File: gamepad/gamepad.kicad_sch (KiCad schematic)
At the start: 33 parts, among them J1 Conn_01x02_Socket, SW1 SW_SPDT, SW2 SW_Push, SW3 SW_Push, SW4 SW_Push, SW5 SW_Push, SW6 SW_Push, SW7 SW_Push, U1 NE555P

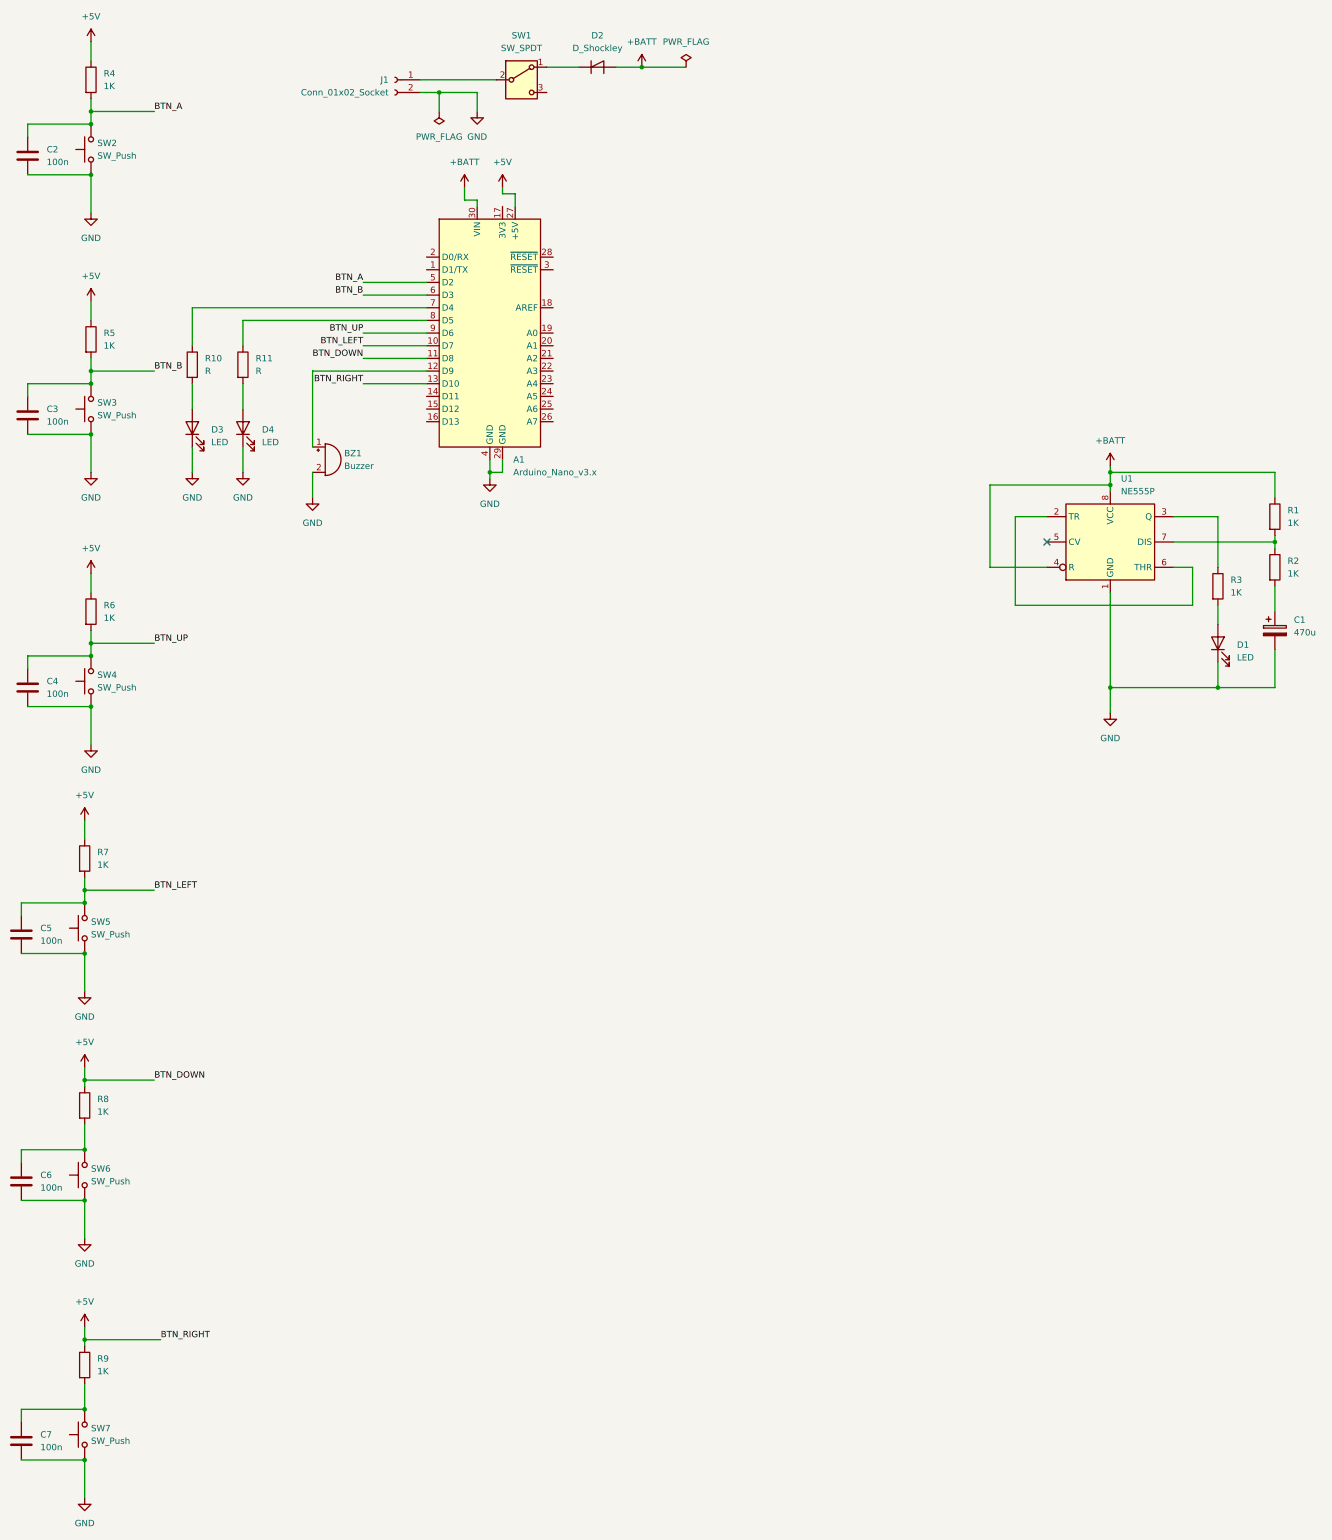
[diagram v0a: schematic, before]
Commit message: schematic is done
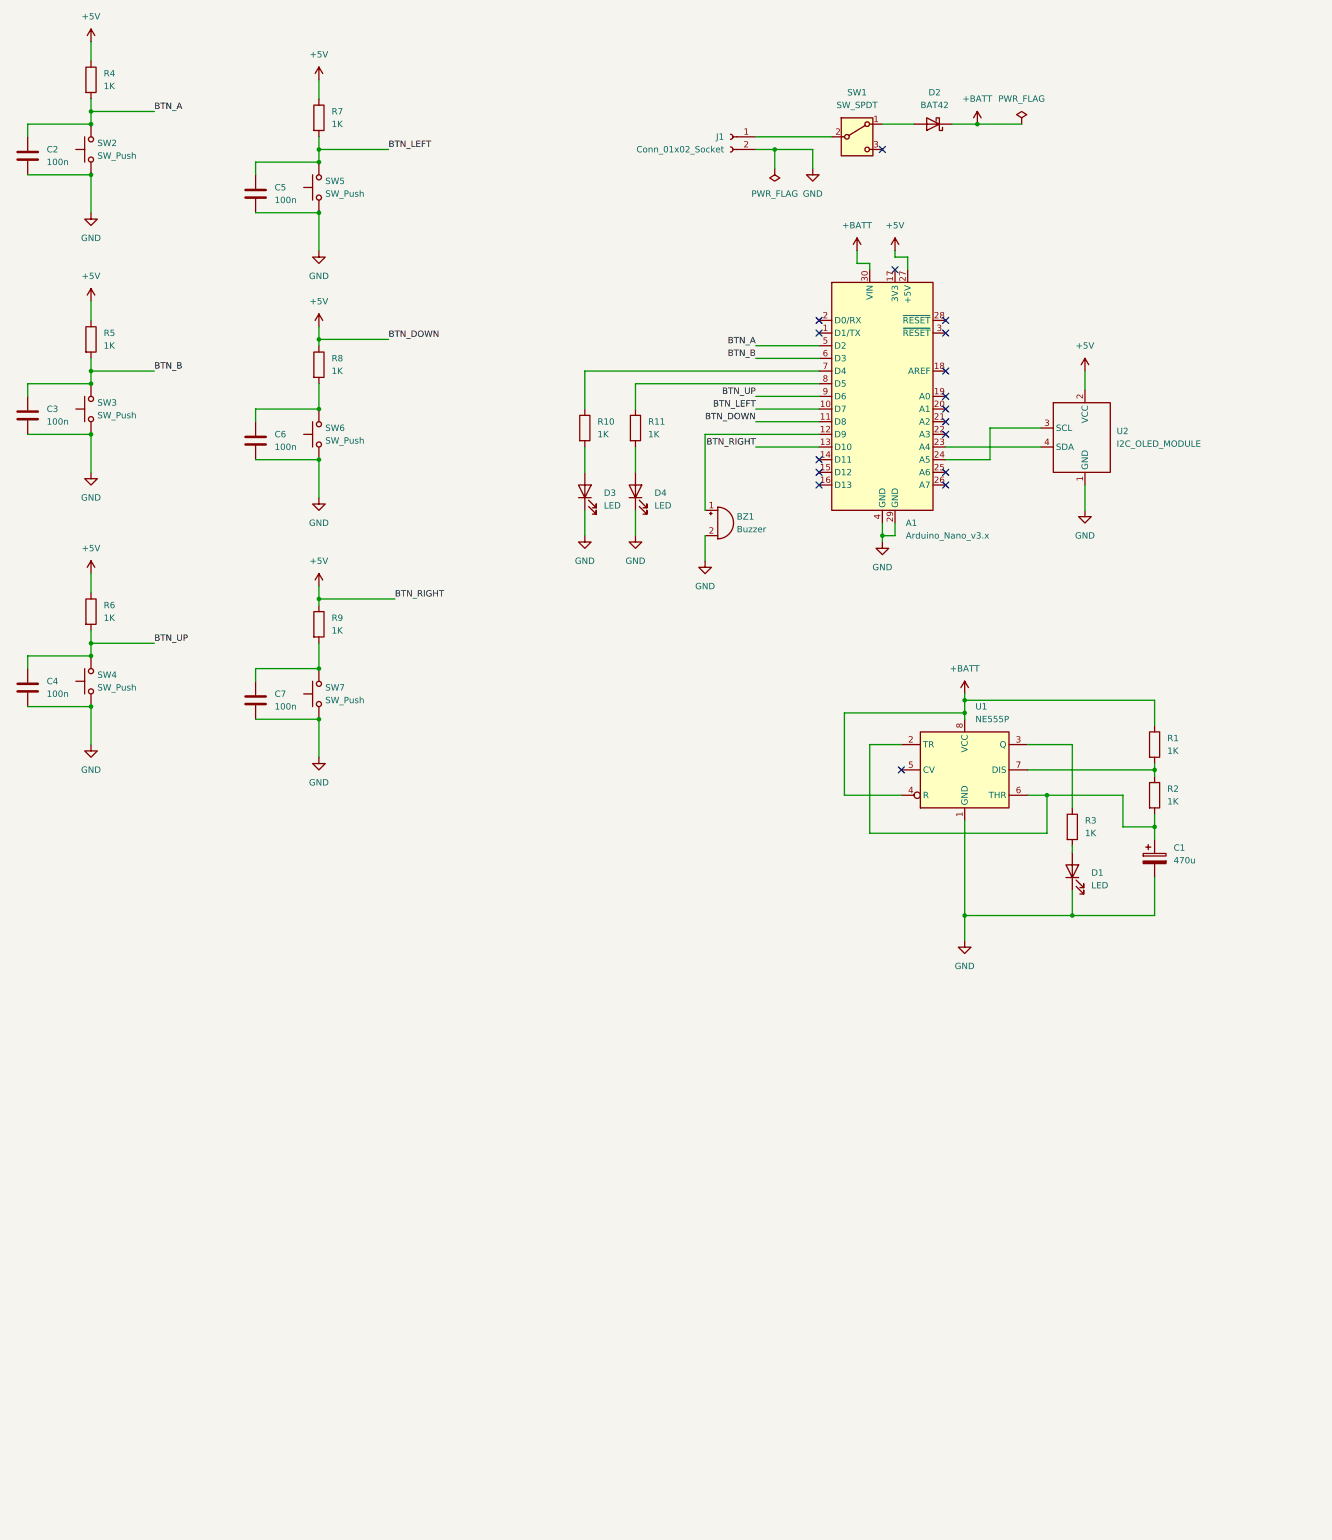
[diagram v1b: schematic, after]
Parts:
- removed D2: D_Shockley, symbol Device:D_Shockley
- added D2: BAT42, Diode_THT:D_DO-35_SOD27_P7.62mm_Horizontal, symbol Diode:BAT42
- added U2: I2C_OLED_MODULE, symbol oled_module:i2c_oled_module
- BZ1: footprint (none) -> Buzzer_Beeper:Buzzer_12x9.5RM7.6
- C2, C3, C4, C5, C6, C7: footprint (none) -> Capacitor_THT:C_Disc_D4.7mm_W2.5mm_P5.00mm
- D1, D3, D4: footprint (none) -> LED_THT:LED_D5.0mm
- J1: footprint (none) -> Connector_Molex:Molex_Micro-Latch_53254-0270_1x02_P2.00mm_Horizontal
- R1, R2, R3, R4, R5, R6, R7, R8, R9: footprint (none) -> Resistor_THT:R_Axial_DIN0207_L6.3mm_D2.5mm_P7.62mm_Horizontal
- R10, R11: value R -> 1K; footprint (none) -> Resistor_THT:R_Axial_DIN0207_L6.3mm_D2.5mm_P7.62mm_Horizontal
- SW2, SW3, SW4, SW5, SW6, SW7: footprint (none) -> Button_Switch_THT:SW_PUSH_6mm
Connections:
- net +5V: now also U2.2 (VCC)
- net +BATT: now also D2.1 (K)
- net GND: now also U2.1 (GND)
- net at C1.1, R2.2: now also U1.2 (TR), U1.6 (THR)
- net at SW1.1 (A): now also D2.2 (A)
- net at A1.23 (A4): now also U2.4 (SDA)
- net at A1.24 (A5): now also U2.3 (SCL)
- no-connect marks 1 -> 17
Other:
- moved on the sheet: A1, BZ1, C1, C5, C6, C7, D1, D3, D4, J1, R1, R10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

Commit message: footprints assigned
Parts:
- C1: footprint (none) -> Capacitor_THT:CP_Radial_D6.3mm_P2.50mm
- SW1: footprint (none) -> spdt_slide_switch:spdt_slide_switch
- U2: footprint (none) -> oled_module:i2c_oled_module
